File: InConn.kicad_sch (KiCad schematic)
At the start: 7 parts, among them J1 2041441-1, J2 USB_C_Receptacle_USB2.0

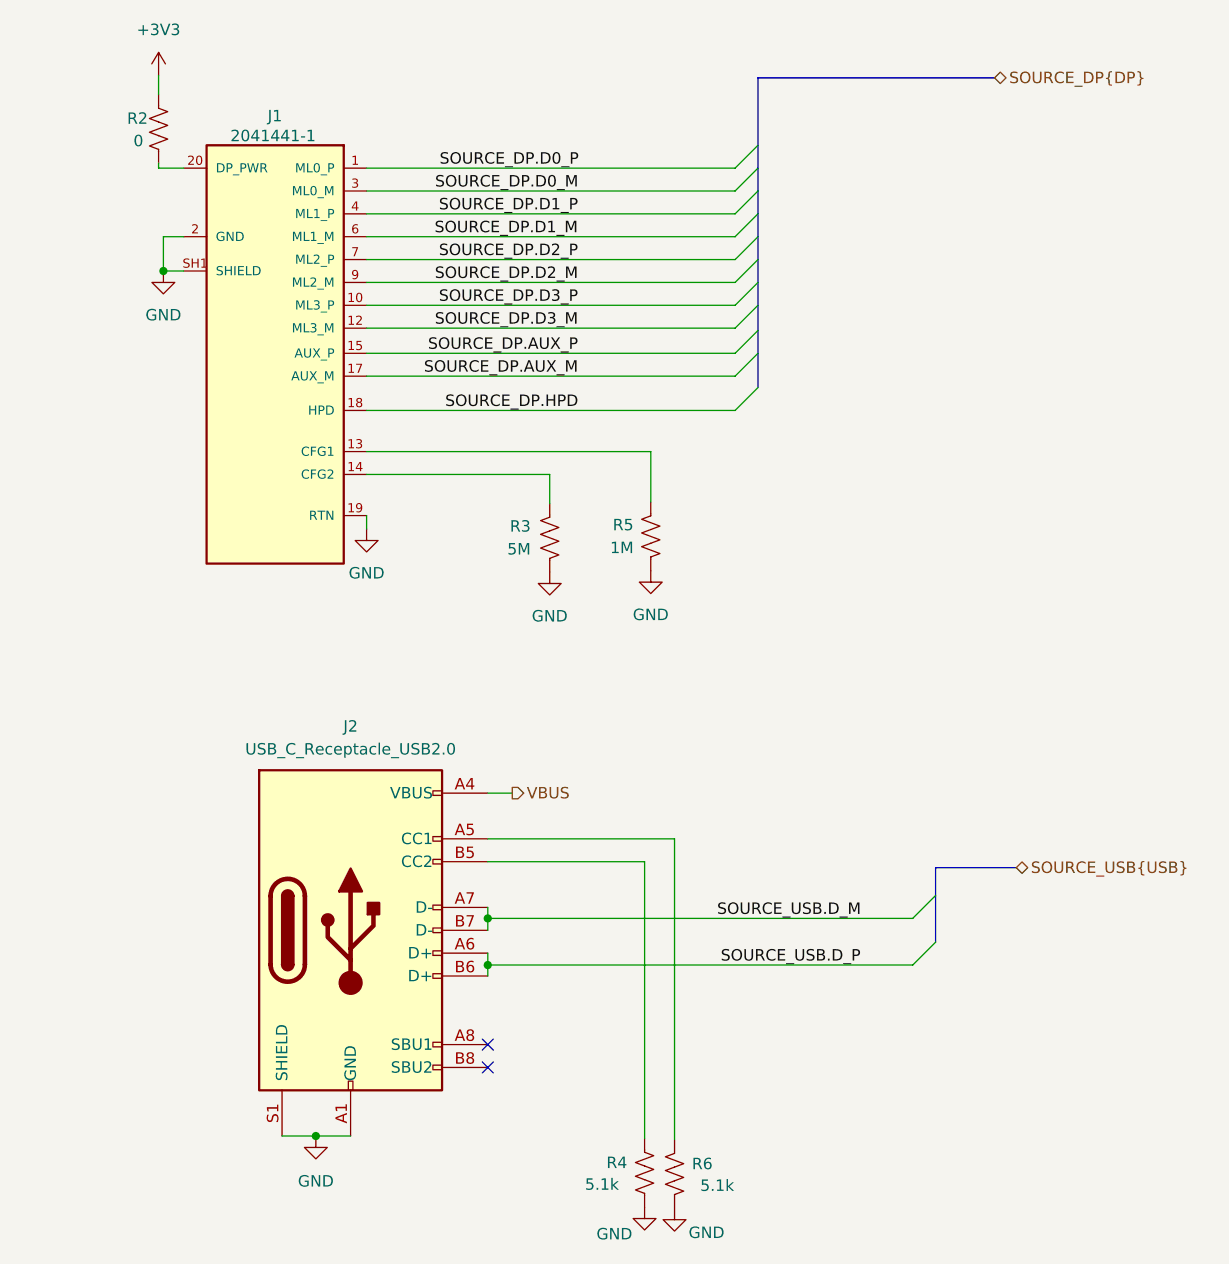
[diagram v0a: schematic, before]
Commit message: Pushing what i have now
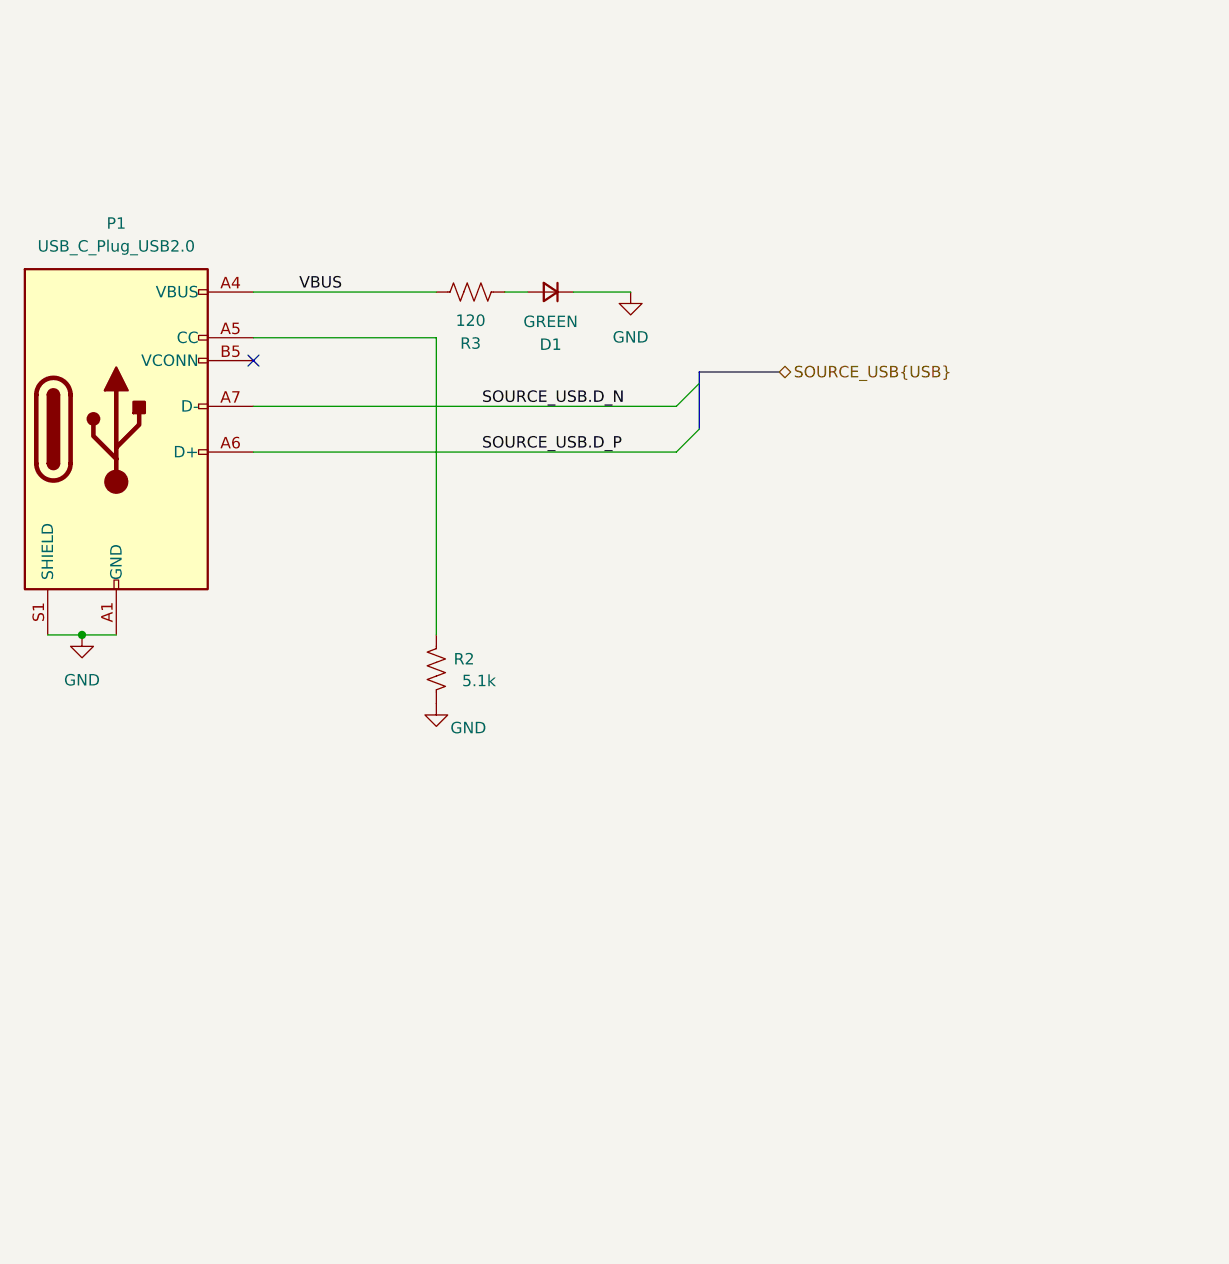
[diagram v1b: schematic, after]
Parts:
- removed J1: 2041441-1, TE_2041441-1, symbol 2041441-1:DP_CONN
- removed J2: USB_C_Receptacle_USB2.0, symbol Connector:USB_C_Receptacle_USB2.0
- removed R2: 0, symbol Device:R_US
- removed R4: 5.1k, symbol Device:R_US
- removed R5: 1M, symbol Device:R_US
- added D1: ${Color}, Diode_SMD:D_0805_2012Metric_Pad1.15x1.40mm_HandSolder, symbol Rockerrobotics:Diodes/754-2043-1-ND
- added P1: USB_C_Plug_USB2.0, Rockerrobotics:AMPHENOL_12402012E212A, symbol Rockerrobotics:Connectors/664-12402012E212ADKR-ND
- R2: renamed from R6; footprint (none) -> Resistor_SMD:R_0603_1608Metric_Pad0.98x0.95mm_HandSolder
- R3: value 5M -> 120; footprint (none) -> Resistor_SMD:R_0603_1608Metric_Pad0.98x0.95mm_HandSolder
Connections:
- net GND: now also D1.1 (K), P1.A1 (GND), P1.A12 (GND), P1.B1 (GND), P1.B12 (GND), P1.S1 (SHIELD); no longer R3.2
- net SOURCE_USB.D_P: now also P1.A6 (D+)
- net VBUS: now also R3.2, P1.A4 (VBUS), P1.A9 (VBUS), P1.B4 (VBUS), P1.B9 (VBUS)
- net at R3.1: now also D1.2 (A)
- net at R2.1: now also P1.A5 (CC)
- new net SOURCE_USB.D_N: P1.A7 (D-)
- no-connect marks 2 -> 1
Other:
- moved on the sheet: R2
